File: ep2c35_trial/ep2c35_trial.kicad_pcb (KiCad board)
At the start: 4 copper layers, 50.3 x 39 mm, 5 parts, among them U1 EP2C5F484

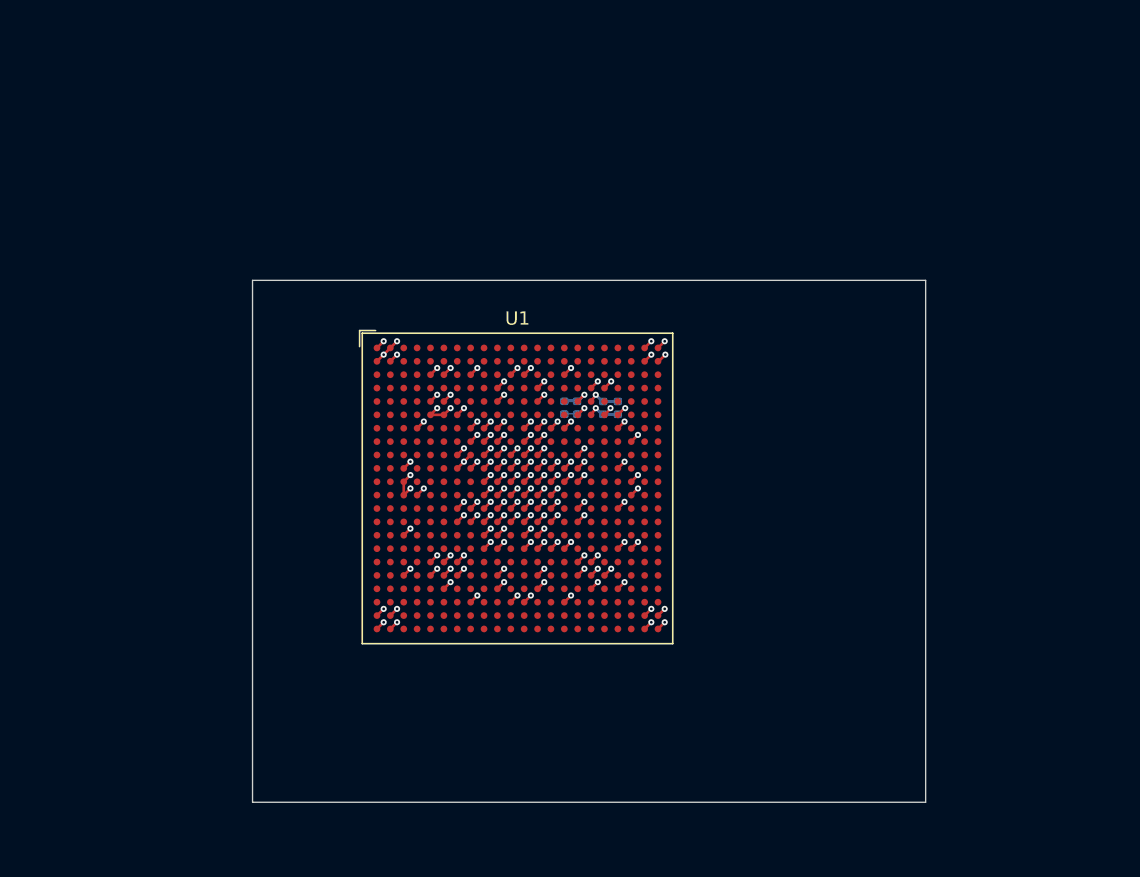
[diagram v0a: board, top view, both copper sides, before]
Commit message: EP2C35 trial. WIP.
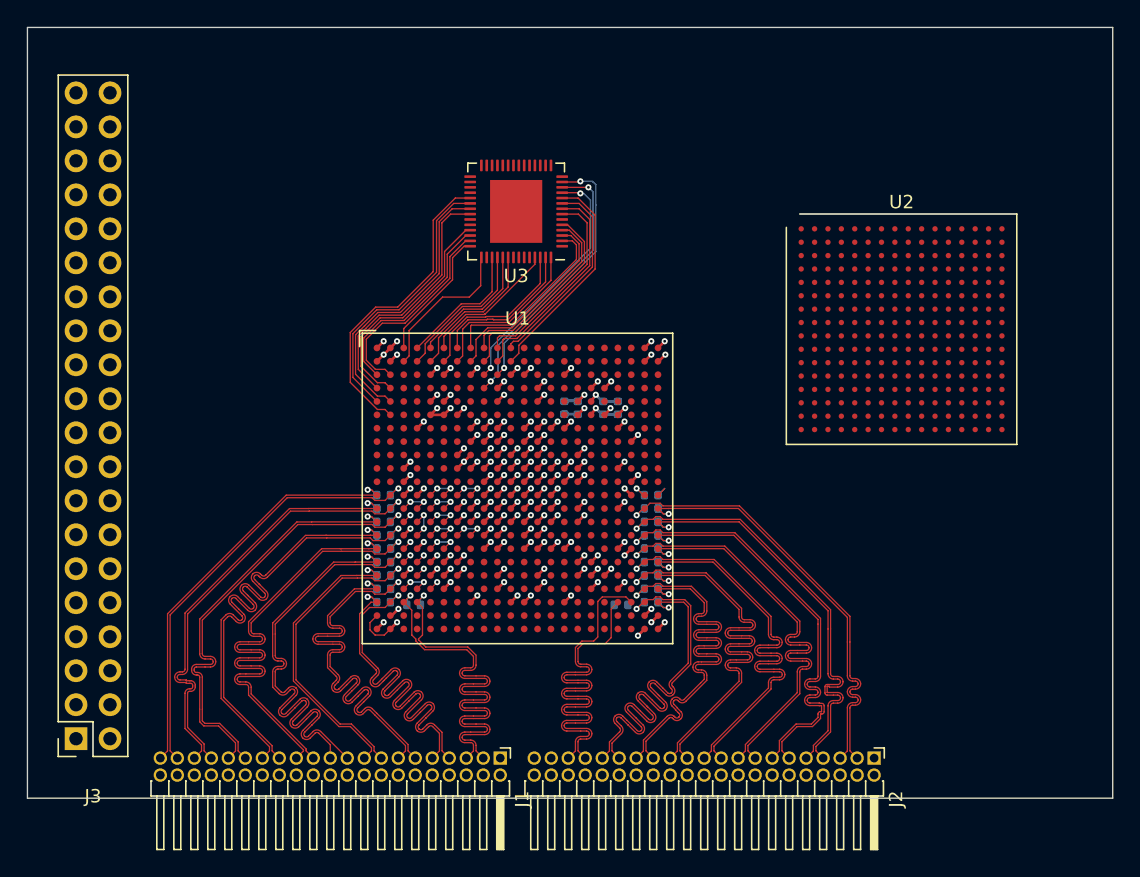
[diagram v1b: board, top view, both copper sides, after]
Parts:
- added J1: Conn_02x21_Odd_Even, Connector_PinHeader_1.27mm:PinHeader_2x21_P1.27mm_Horizontal, F.Cu at (143.2, 101.7)
- added J2: Conn_02x21_Odd_Even, Connector_PinHeader_1.27mm:PinHeader_2x21_P1.27mm_Horizontal, F.Cu at (171.2, 101.7)
- added J3: 3M_8540-4500PL, logic_analyzer:3M_8540-4500PL, F.Cu at (111.5, 100.2)
- added R11: 100, Resistor_SMD:R_0402_1005Metric, B.Cu at (154.5, 83.0)
- added R12: 100, Resistor_SMD:R_0402_1005Metric, B.Cu at (154.5, 84.0)
- added R13: 100, Resistor_SMD:R_0402_1005Metric, B.Cu at (154.5, 85.0)
- added R14: 100, Resistor_SMD:R_0402_1005Metric, B.Cu at (154.5, 86.0)
- added R15: 100, Resistor_SMD:R_0402_1005Metric, B.Cu at (154.5, 87.0)
- added R16: 100, Resistor_SMD:R_0402_1005Metric, B.Cu at (154.5, 88.0)
- added R17: 100, Resistor_SMD:R_0402_1005Metric, B.Cu at (154.5, 89.0)
- added R18: 100, Resistor_SMD:R_0402_1005Metric, B.Cu at (154.5, 90.0)
- added R19: 100, Resistor_SMD:R_0402_1005Metric, B.Cu at (152.2, 90.2)
- added R20: 100, Resistor_SMD:R_0402_1005Metric, B.Cu at (154.5, 82.0)
- added R21: 100, Resistor_SMD:R_0402_1005Metric, B.Cu at (134.5, 90.0)
- added R22: 100, Resistor_SMD:R_0402_1005Metric, B.Cu at (134.5, 89.0)
- added R23: 100, Resistor_SMD:R_0402_1005Metric, B.Cu at (134.5, 88.0)
- added R24: 100, Resistor_SMD:R_0402_1005Metric, B.Cu at (134.5, 87.0)
- added R25: 100, Resistor_SMD:R_0402_1005Metric, B.Cu at (134.5, 86.0)
- added R26: 100, Resistor_SMD:R_0402_1005Metric, B.Cu at (134.5, 85.0)
- added R27: 100, Resistor_SMD:R_0402_1005Metric, B.Cu at (134.5, 84.0)
- added R28: 100, Resistor_SMD:R_0402_1005Metric, B.Cu at (134.5, 83.0)
- added R29: 100, Resistor_SMD:R_0402_1005Metric, B.Cu at (136.7, 90.2)
- added R30: 100, Resistor_SMD:R_0402_1005Metric, B.Cu at (134.5, 82.0)
- added U2: XC6SLX16-FTG256, Package_BGA:Xilinx_FTG256, F.Cu at (173.2, 69.6)
- added U3: FT600Q-B-T, logic_analyzer:QFN-56-1EP_7x7mm_P0.4mm_FT600Q, F.Cu at (144.4, 60.8)
- moved C1 0.05 mm to (149.0, 75.5)
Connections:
- U1 pad A10: unconnected-(U1-PadA10) -> /FT_WR_N
- U1 pad A11: unconnected-(U1-PadA11) -> /FT_OE_N
- U1 pad A2: +2V5 -> +3.3V
- U1 pad A21: +2V5 -> +3.3V
- U1 pad A3: unconnected-(U1-PadA3) -> /FT_DATA7
- U1 pad A4: unconnected-(U1-PadA4) -> /FT_DATA8
- U1 pad A5: unconnected-(U1-PadA5) -> /FT_DATA10
- U1 pad A6: unconnected-(U1-PadA6) -> /FT_DATA12
- U1 pad A7: unconnected-(U1-PadA7) -> /FT_DATA14
- U1 pad A8: unconnected-(U1-PadA8) -> /FT_BE0
- U1 pad A9: unconnected-(U1-PadA9) -> /FT_TXE_N
- U1 pad B1: +2V5 -> +3.3V
- U1 pad B10: unconnected-(U1-PadB10) -> /FT_RD_N
- U1 pad B11: unconnected-(U1-PadB11) -> /FT_RESET_N
- U1 pad B22: +2V5 -> +3.3V
- U1 pad B3: unconnected-(U1-PadB3) -> /FT_CLK
- U1 pad B4: unconnected-(U1-PadB4) -> /FT_DATA9
- U1 pad B5: unconnected-(U1-PadB5) -> /FT_DATA11
- U1 pad B6: unconnected-(U1-PadB6) -> /FT_DATA13
- U1 pad B7: unconnected-(U1-PadB7) -> /FT_DATA15
- U1 pad B8: unconnected-(U1-PadB8) -> /FT_BE1
- U1 pad B9: unconnected-(U1-PadB9) -> /FT_RXF_N
- U1 pad C1: unconnected-(U1-PadC1) -> /FT_DATA5
- U1 pad C10: unconnected-(U1-PadC10) -> /FT_GPIO1
- U1 pad C11: +2V5 -> +3.3V
- U1 pad C12: +2V5 -> +3.3V
- U1 pad C2: unconnected-(U1-PadC2) -> /FT_DATA6
- U1 pad C6: +2V5 -> +3.3V
- U1 pad C9: unconnected-(U1-PadC9) -> /FT_WAKEUP_N
- U1 pad D1: unconnected-(U1-PadD1) -> /FT_DATA3
- U1 pad D17: +2V5 -> +3.3V
- U1 pad D2: unconnected-(U1-PadD2) -> /FT_DATA4
- U1 pad D9: unconnected-(U1-PadD9) -> /FT_GPIO0
- U1 pad E1: unconnected-(U1-PadE1) -> /FT_DATA1
- U1 pad E10: +2V5 -> +3.3V
- U1 pad E13: +2V5 -> +3.3V
- U1 pad E2: unconnected-(U1-PadE2) -> /FT_DATA2
- U1 pad F2: unconnected-(U1-PadF2) -> /FT_DATA0
- U1 pad G14: +2V5 -> +3.3V
- U1 pad G19: +2V5 -> +3.3V
- U1 pad G9: +2V5 -> +3.3V
- U1 pad J16: +2V5 -> +3.3V
- U1 pad J7: +2V5 -> +3.3V
- U1 pad L20: +2V5 -> +3.3V
- U1 pad L3: +2V5 -> +3.3V
- U1 pad M1: unconnected-(U1-PadM1) -> /LVDS_RX_CLK0_P
- U1 pad M2: unconnected-(U1-PadM2) -> /LVDS_RX_CLK0_N
- U1 pad M21: unconnected-(U1-PadM21) -> /LVDS_RX_CLK1_N
- U1 pad M22: unconnected-(U1-PadM22) -> GNDD
- U1 pad M5: unconnected-(U1-PadM5) -> Net-(U1-PadM5)
- U1 pad M6: unconnected-(U1-PadM6) -> Net-(U1-PadM5)
- U1 pad M7: unconnected-(U1-PadM7) -> Net-(U1-PadM7)
- U1 pad M8: unconnected-(U1-PadM8) -> Net-(U1-PadM7)
- U1 pad N1: unconnected-(U1-PadN1) -> /LVDS_RX_DATA0_0_P
- U1 pad N2: unconnected-(U1-PadN2) -> /LVDS_RX_DATA0_0_N
- U1 pad N21: unconnected-(U1-PadN21) -> /LVDS_RX_DATA1_7_N
- U1 pad N22: unconnected-(U1-PadN22) -> /LVDS_RX_DATA1_7_P
- U1 pad N3: unconnected-(U1-PadN3) -> Net-(U1-PadN3)
- U1 pad N4: unconnected-(U1-PadN4) -> Net-(U1-PadN3)
- U1 pad N5: unconnected-(U1-PadN5) -> Net-(U1-PadN5)
- U1 pad N6: unconnected-(U1-PadN6) -> Net-(U1-PadN5)
- U1 pad P1: unconnected-(U1-PadP1) -> /LVDS_RX_DATA0_1_P
- U1 pad P2: unconnected-(U1-PadP2) -> /LVDS_RX_DATA0_1_N
- U1 pad P21: unconnected-(U1-PadP21) -> /LVDS_RX_DATA1_6_N
- U1 pad P22: unconnected-(U1-PadP22) -> /LVDS_RX_DATA1_6_P
- U1 pad P4: unconnected-(U1-PadP4) -> Net-(U1-PadP4)
- U1 pad P5: unconnected-(U1-PadP5) -> Net-(U1-PadP5)
- U1 pad P6: unconnected-(U1-PadP6) -> Net-(U1-PadP5)
- U1 pad R1: unconnected-(U1-PadR1) -> /LVDS_RX_DATA0_2_P
- U1 pad R2: unconnected-(U1-PadR2) -> /LVDS_RX_DATA0_2_N
- U1 pad R21: unconnected-(U1-PadR21) -> /LVDS_RX_DATA1_5_N
- U1 pad R22: unconnected-(U1-PadR22) -> /LVDS_RX_DATA1_5_P
- U1 pad R4: unconnected-(U1-PadR4) -> Net-(U1-PadP4)
- U1 pad R5: unconnected-(U1-PadR5) -> Net-(U1-PadR5)
- U1 pad R6: unconnected-(U1-PadR6) -> Net-(U1-PadR5)
- U1 pad R7: unconnected-(U1-PadR7) -> Net-(U1-PadR7)
- U1 pad R8: unconnected-(U1-PadR8) -> Net-(U1-PadR7)
- U1 pad T1: unconnected-(U1-PadT1) -> /LVDS_RX_DATA0_3_P
- U1 pad T2: unconnected-(U1-PadT2) -> /LVDS_RX_DATA0_3_N
- U1 pad T21: unconnected-(U1-PadT21) -> /LVDS_RX_DATA1_4_N
- U1 pad T22: unconnected-(U1-PadT22) -> /LVDS_RX_DATA1_4_P
- U1 pad T5: unconnected-(U1-PadT5) -> Net-(U1-PadT5)
- U1 pad T6: unconnected-(U1-PadT6) -> Net-(U1-PadT5)
- U1 pad U1: unconnected-(U1-PadU1) -> /LVDS_RX_DATA0_4_P
- U1 pad U2: unconnected-(U1-PadU2) -> /LVDS_RX_DATA0_4_N
- U1 pad U21: unconnected-(U1-PadU21) -> /LVDS_RX_DATA1_3_N
- U1 pad U22: unconnected-(U1-PadU22) -> /LVDS_RX_DATA1_3_P
- U1 pad V1: unconnected-(U1-PadV1) -> /LVDS_RX_DATA0_5_P
- U1 pad V2: unconnected-(U1-PadV2) -> /LVDS_RX_DATA0_5_N
- U1 pad V21: unconnected-(U1-PadV21) -> /LVDS_RX_DATA1_2_N
- U1 pad V22: unconnected-(U1-PadV22) -> /LVDS_RX_DATA1_2_P
- U1 pad W1: unconnected-(U1-PadW1) -> /LVDS_RX_DATA0_6_P
- U1 pad W2: unconnected-(U1-PadW2) -> /LVDS_RX_DATA0_6_N
- U1 pad W21: unconnected-(U1-PadW21) -> /LVDS_RX_DATA1_1_N
- U1 pad W22: unconnected-(U1-PadW22) -> /LVDS_RX_DATA1_1_P
- U1 pad W3: unconnected-(U1-PadW3) -> Net-(U1-PadW3)
- U1 pad W4: unconnected-(U1-PadW4) -> Net-(U1-PadW3)
- U1 pad Y1: unconnected-(U1-PadY1) -> /LVDS_RX_DATA0_7_P
- U1 pad Y19: unconnected-(U1-PadY19) -> /LVDS_RX_FCLK1_N
- U1 pad Y2: unconnected-(U1-PadY2) -> /LVDS_RX_DATA0_7_N
- U1 pad Y20: unconnected-(U1-PadY20) -> /LVDS_RX_FCLK1_P
- U1 pad Y21: unconnected-(U1-PadY21) -> /LVDS_RX_DATA1_0_N
- U1 pad Y22: unconnected-(U1-PadY22) -> /LVDS_RX_DATA1_0_P
- U1 pad Y3: unconnected-(U1-PadY3) -> /LVDS_RX_FCLK0_P
- U1 pad Y4: unconnected-(U1-PadY4) -> /LVDS_RX_FCLK0_N
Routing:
- net /LVDS_RX_DATA0_2_N: track 0.00 -> 37.8 mm, vias 0 -> 1
- net /LVDS_RX_DATA0_2_P: track 0.00 -> 37.2 mm, vias 0 -> 1
- net /LVDS_RX_DATA0_3_N: track 0.00 -> 36.9 mm, vias 0 -> 1
- net /LVDS_RX_DATA0_3_P: track 0.00 -> 36.3 mm, vias 0 -> 1
- net /LVDS_RX_DATA0_4_N: track 0.00 -> 36.1 mm, vias 0 -> 1
- net /LVDS_RX_DATA0_4_P: track 0.00 -> 35.0 mm, vias 0 -> 1
- net /LVDS_RX_DATA1_6_N: track 0.00 -> 33.6 mm, vias 0 -> 1
- net /LVDS_RX_DATA0_1_N: track 0.00 -> 33.5 mm, vias 0 -> 1
- net /LVDS_RX_DATA1_7_N: track 0.00 -> 33.5 mm, vias 0 -> 1
- net /LVDS_RX_DATA1_5_N: track 0.00 -> 33.5 mm, vias 0 -> 1
- net /LVDS_RX_DATA0_0_N: track 0.00 -> 33.4 mm, vias 0 -> 1
- net /LVDS_RX_DATA1_4_N: track 0.00 -> 33.4 mm, vias 0 -> 1
- net /LVDS_RX_DATA1_3_N: track 0.00 -> 33.3 mm, vias 0 -> 1
- net /LVDS_RX_DATA1_2_N: track 0.00 -> 33.3 mm, vias 0 -> 1
- net /LVDS_RX_DATA1_0_N: track 0.00 -> 33.3 mm, vias 0 -> 1
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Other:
- board size 50.3 x 39 mm -> 81.1 x 57.6 mm
